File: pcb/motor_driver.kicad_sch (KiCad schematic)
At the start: 5 parts, among them J1 Brushed DC Motor, U1 DRV8212P

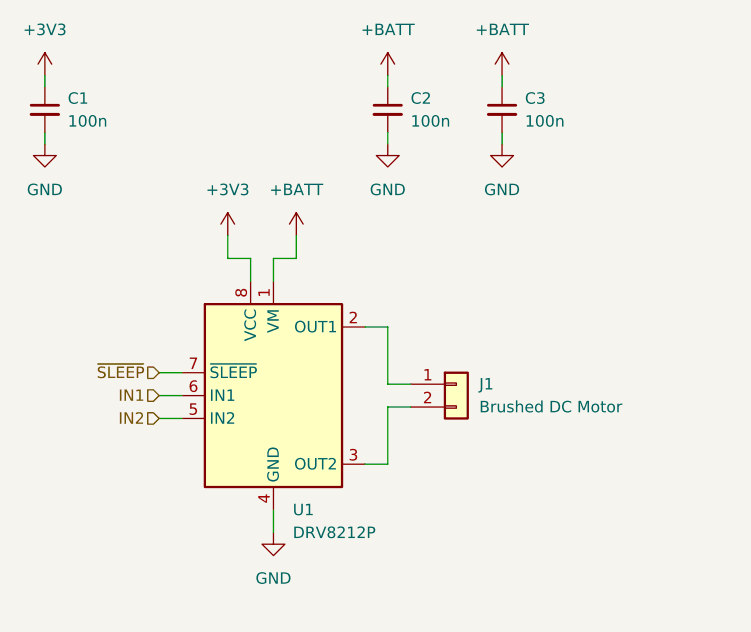
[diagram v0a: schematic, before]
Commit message: Finish design
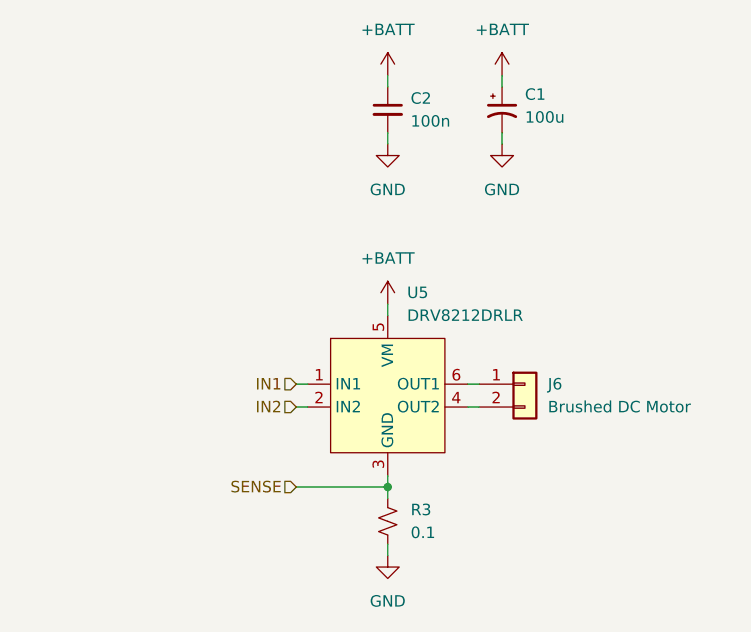
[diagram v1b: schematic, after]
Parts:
- removed C1, C3: 100n, symbol Device:C_Small
- removed J1: Brushed DC Motor, symbol Connector_Generic:Conn_01x02
- removed U1: DRV8212P, Package_SON:WSON-8-1EP_2x2mm_P0.5mm_EP0.9x1.6mm_ThermalVias, symbol Driver_Motor:DRV8212P
- added C1: 100u, symbol Device:C_Polarized_Small_US
- added J6: Brushed DC Motor, symbol Connector_Generic:Conn_01x02
- added R3: 0.1, symbol Device:R_Small_US
- added U5: DRV8212DRLR, Package_TO_SOT_SMD:SOT-563, symbol DRV8212DRLR:DRV8212DRLR
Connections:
- net +BATT: now also C1.1, U5.5 (VM)
- net GND: now also C1.2, R3.2
- net IN1: now also U5.1 (IN1)
- net IN2: now also U5.2 (IN2)
- new net: J6.1 (Pin_1), U5.6 (OUT1)
- new net: J6.2 (Pin_2), U5.4 (OUT2)
- new net SENSE: R3.1, U5.3 (GND)
